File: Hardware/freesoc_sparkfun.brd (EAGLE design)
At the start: 116.8 x 55.9 mm, 92 parts, among them J1 5.5x2.1mm Barrel, U1 CY8C5888AXI-LP096, U2 AP2202-ADJ, U3 AP2202-ADJ, U4 AP2202-ADJ, U5 AP2202-ADJ, U6 AP2202-ADJ, U7 CY8C5868LTI-LP039

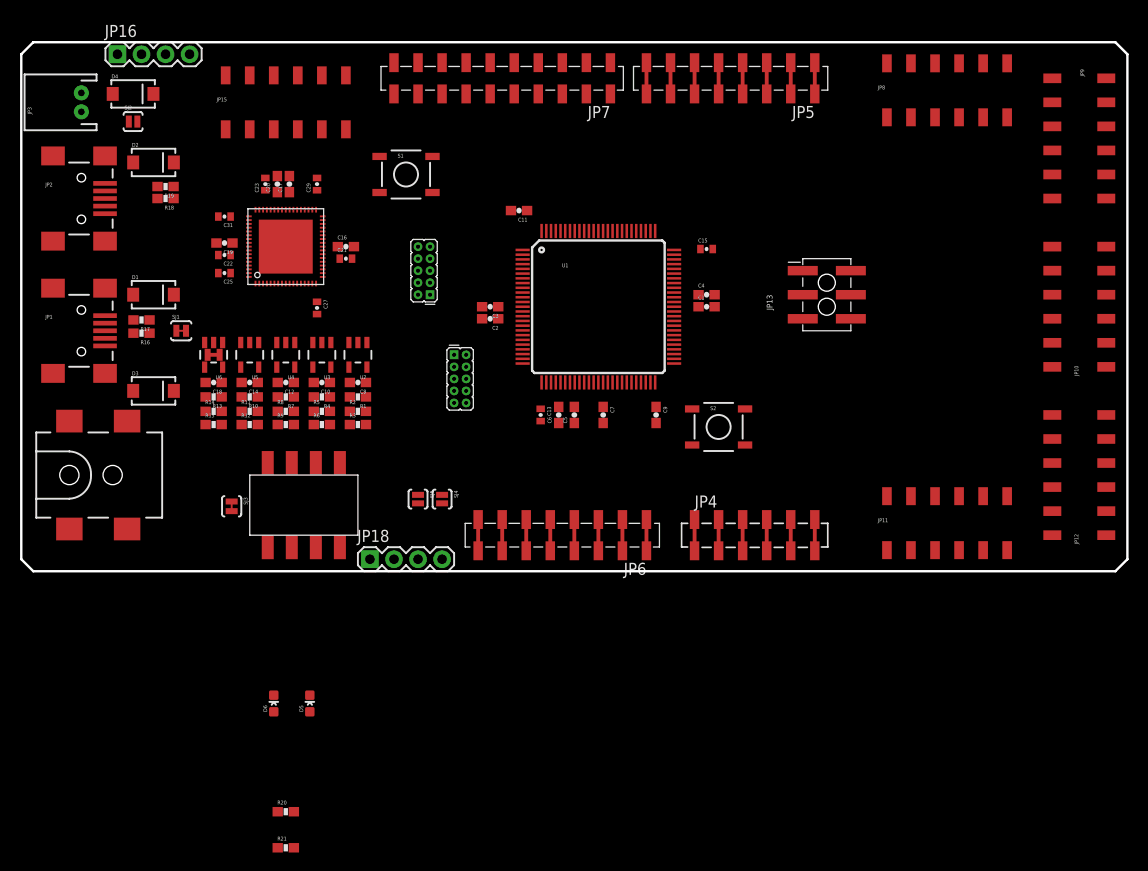
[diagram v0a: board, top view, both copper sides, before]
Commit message: Routed, ready for review.
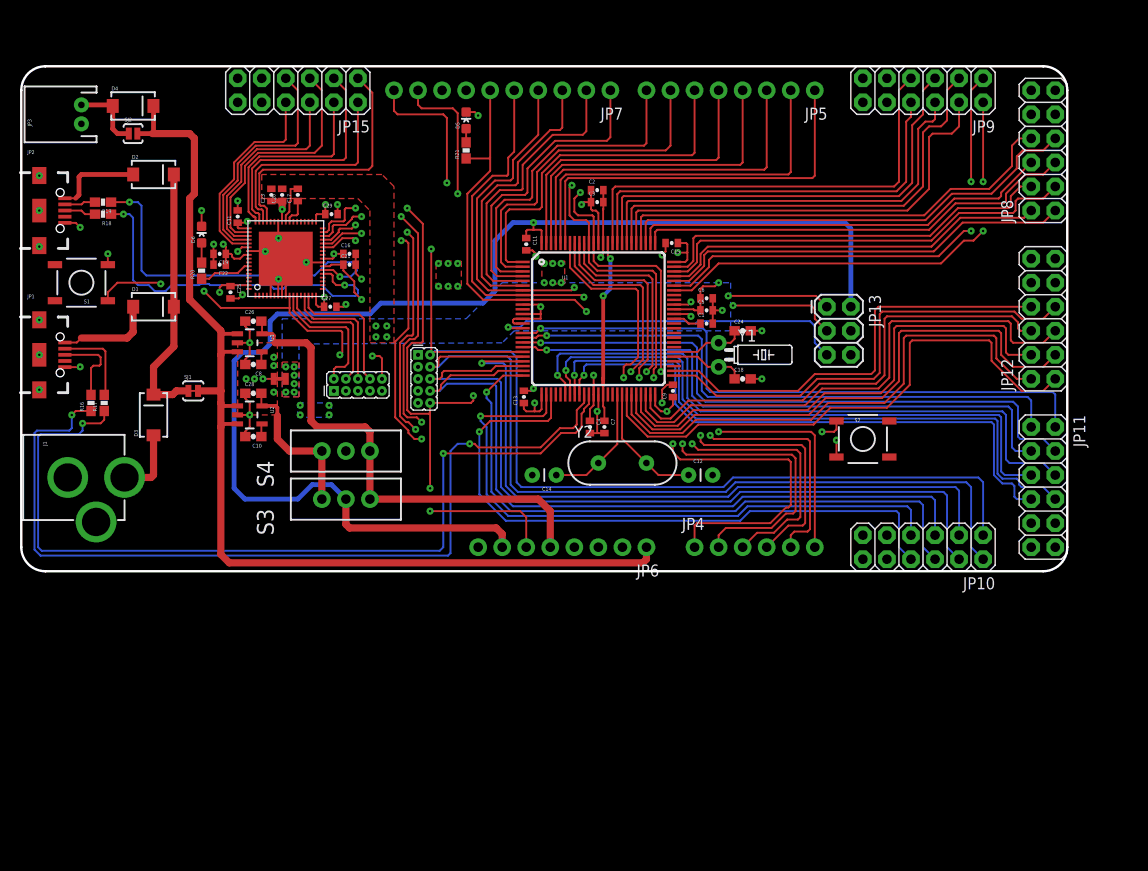
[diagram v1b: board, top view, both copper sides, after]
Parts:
- removed JP16, JP18: (no value), SparkFun-Connectors:1X04
- removed R1, R10, R13, R4, R7: 5.62k, SparkFun-Resistors:0603-RES
- removed R11, R14, R2, R5, R8: 3.40k, SparkFun-Resistors:0603-RES
- removed R12, R15, R3, R6, R9: 4.12k, SparkFun-Resistors:0603-RES
- removed SJ3: JUMPER-PAD-2-NC_BY_TRACE, SparkFun-Passives:PAD-JUMPER-2-NC_BY_TRACE_YES_SILK
- removed SJ4, SJ5: JUMPER-PAD-2-NOYES_SILK, SparkFun-Passives:PAD-JUMPER-2-NO_YES_SILK
- removed U$1: 4-POS-DIP, SparkFun-Electromechanical:4-POS-DIP-SMD
- removed U4, U5, U6: AP2202-ADJ, SparkFun-PowerIC:SOT23-5
- added C24: 22pF, SparkFun-Capacitors:0603-CAP
- added C26, C28: 2.2uF, SparkFun-Capacitors:0603-CAP
- added S3, S4: (no value), SparkFun-Electromechanical:SWITCH-SPDT
- added Y1: 32.768kHz, SparkFun-FreqCtrl:TC26H
- added Y2: (no value), SparkFun-FreqCtrl:HC49US
- C1, C11, C16, C17, C19, C2, C20, C3, C4, C5, C6, C7, C9: device SparkFun-Capacitors:0603-CAP -> SparkFun-Capacitors:0402-CAP
- C10, C8: value 2.2uF -> 470pF
- C12, C14: value 2.2uF -> (none); device SparkFun-Capacitors:0603-CAP -> SparkFun-Capacitors:CAP-PTH-SMALL
- C18: value 2.2uF -> 22pF
- J1: value 5.5x2.1mm Barrel -> POWER_JACKPTH; device SparkFun-Connectors:POWER_JACK_SMD -> SparkFun-Connectors:POWER_JACK_PTH
- JP1, JP2: value USBSMD -> MicroB; device SparkFun-Connectors:USB-MINIB -> SparkFun-Connectors:USB-B-MICRO-SMD_V03
- JP10, JP11, JP12, JP15, JP8, JP9: value M06X2FEMALE-SMT -> 2X6 FEMALE; device SparkFun-Connectors:2X6_SMD -> SparkFun-Connectors:2X6
- JP13: device SparkFun-Connectors:2X3_SMT_POSTS -> SparkFun-Connectors:2X3
- JP4: device SparkFun-Connectors:1X06_SMD_STRAIGHT_COMBO -> SparkFun-Connectors:1X06_NO_SILK
- JP5, JP6: device SparkFun-Connectors:1X08_SMD_COMBINED -> SparkFun-Connectors:1X08_NO_SILK
- JP7: value M10SMD_COMBO-FEMALE -> M10NO_SILK_PTH_FEMALE; device SparkFun-Connectors:1X10_SMD_COMBINED -> SparkFun-Connectors:1X10_NO_SILK
- U1: value CY8C5888AXI-LP096 -> CY8C5868AXI-LP035
- U2: value AP2202-ADJ -> MIC5219 5V
- U3: value AP2202-ADJ -> MIC5219 3.3V
- moved R21 76.1 mm to (47.0, 44.5), turned to 90 degrees
- moved D5 63.8 mm to (47.0, 47.6)
- moved R20 57.8 mm to (19.1, 31.8), turned to 90 degrees
- moved C18 55.9 mm to (76.2, 20.3), turned to 0 degrees
- moved D6 50.1 mm to (19.1, 35.6)
- moved C12 43.7 mm to (70.5, 10.2), turned to 0 degrees
- moved S1 36.1 mm to (6.35, 30.5), turned to 180 degrees
- moved C14 33.8 mm to (56.5, 10.2)
- moved JP10 25.0 mm to (101.6, 3.81), turned to 180 degrees
- moved C6 19.9 mm to (72.4, 28.8), turned to 0 degrees
- moved C4 18.6 mm to (60.1, 15.2), turned to 270 degrees
- moved JP8 18.0 mm to (109.2, 38.1), turned to 90 degrees
- moved C5 17.8 mm to (72.4, 27.6), turned to 0 degrees
- moved C2 17.7 mm to (60.8, 40.3), turned to 0 degrees
- moved JP14 16.9 mm to (39.4, 19.1), turned to 90 degrees
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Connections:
- net N$18 renamed PSOC_D+_PAD
- net N$19 renamed DEBUG_D-_PAD
- net N$22 renamed DEBUG_D+_PAD
- net N$3 renamed PSOC_D-_PAD
- removed net ADJ2: R1.2, R2.1, R3.1, U2.4
- removed net ADJ3: R4.2, R5.1, R6.1, U3.4
- removed net ADJ4: R7.2, R8.1, R9.1, U4.4
- removed net ADJ5: R10.2, R11.1, R12.1, U5.4
- removed net ADJ6: R13.2, R14.1, R15.1, U6.4
- removed net DEBUG_D+: JP2.D+, R18.2
- removed net DEBUG_D-: JP2.D-, R19.2
- removed net N$24: R20.1
- removed net N$31: SJ4.1, U7.38
- removed net N$32: SJ5.1, U7.39
- removed net PSOC_D+: JP1.D+, R16.2
- removed net PSOC_D-: JP1.D-, R17.2
- removed net SW2: R3.2, U$1.4
- removed net SW3: R6.2, U$1.3
- removed net SW4: R9.2, U$1.2
- removed net SW5: R12.2, U$1.1
- removed net SW6: R15.2, SJ3.1
- removed net VDDD/VDDA: C18.1, C19.1, C2.1, C20.1, C21.1, C22.1, C23.1, C25.1, C27.1, C3.1, C31.1, C4.1, C5.1, C6.1, JP14.1, JP15.10, JP15.9, JP16.2, JP6.4, JP6.5, R13.1, U1.37, U1.65, U1.88, U6.5, U7.17, U7.24, U7.44, U7.52, U7.59, U7.67
- removed net VDDIO_0: C14.1, C15.1, JP8.10, JP8.9, JP9.10, JP9.9, R10.1, U1.75, U5.5
- removed net VDDIO_1: C12.1, C13.1, C29.1, JP10.10, JP10.9, JP11.10, JP11.9, JP17.1, R7.1, U1.26, U4.5, U7.35
- removed net VDDIO_2: C10.1, C11.1, JP13.2, JP6.7, R4.1, U1.100, U3.5
- removed net VDDIO_3: C8.1, C9.1, JP12.10, JP12.9, JP18.2, R1.1, U1.50, U2.5
- new net 3.3V: C26.2, JP6.5, S3.3, S4.3, U3.5
- new net 5V: C20.1, C23.1, C28.2, C5.1, C6.1, JP6.4, S3.1, S4.1, U1.65, U2.5, U7.44
- new net DEBUG_D+_BUS: JP2.D+1, R18.2
- new net DEBUG_D-_BUS: JP2.D-1, R19.2
- new net DEBUG_LED: R20.1, U7.62
- new net N$1: C8.1, U3.4
- new net N$2: C10.1, U2.4
- new net PSOC_D+_BUS: JP1.D+1, R16.2
- new net PSOC_D-_BUS: JP1.D-1, R17.2
- new net VDDIO: C13.1, C15.1, C19.1, C2.1, C21.1, C22.1, C25.1, C27.1, C29.1, C3.1, C31.1, C4.1, C9.1, JP10.10, JP10.9, JP11.10, JP11.9, JP12.10, JP12.9, JP14.1, JP15.10, JP15.9, JP17.1, JP8.10, JP8.9, JP9.10, JP9.9, S4.2, U1.26, U1.37, U1.50, U1.75, U1.88, U7.17, U7.24, U7.35, U7.52, U7.59, U7.67
- new net VDDIO_ARDUINO: C11.1, JP13.2, JP6.7, S3.2, U1.100
- net A0: now also U1.94; no longer U1.89
- net A1: now also U1.93; no longer U1.90
- net A2: now also U1.92; no longer U1.91
- net A3: now also U1.91; no longer U1.92
- net A4: now also JP7.10, U1.90; no longer JP7.10A, JP7.10B, U1.93
- net A5: now also JP7.9, U1.89; no longer JP7.9A, JP7.9B, U1.94
- net AGND: now also C17.2, C20.2, C23.2, U7.43
- net D0: now also U1.95; no longer U1.99
- net D1: now also U1.96; no longer U1.1
- net D10: now also JP7.3, U1.6; no longer JP7.3A, JP7.3B, U1.2
- net D11: now also JP7.4, U1.7; no longer JP7.4A, JP7.4B, U1.8
- net D12: now also JP7.5, U1.8; no longer JP7.5A, JP7.5B, U1.7
- net D13: now also JP7.6; no longer JP7.6A, JP7.6B
- net D2: now also U1.97; no longer U1.98
- net D3: now also U1.98; no longer U1.5
- net D4: now also U1.99; no longer U1.95
- net D5: now also U1.1; no longer U1.6
- net D6: now also U1.2; no longer U1.3
- net D7: now also U1.3; no longer U1.97
- net D8: now also JP7.1, U1.4; no longer JP7.1A, JP7.1B, U1.96
- net D9: now also JP7.2, U1.5; no longer JP7.2A, JP7.2B, U1.4
- net DEBUG_I2C0_SCL: no longer JP16.4
- net DEBUG_I2C0_SDA: no longer JP16.3
- net GND: now also C24.2, C26.1, C28.1, J1.GNDBREAK, JP1.GND1, JP1.SHIELD1, JP1.SHIELD2, JP1.SHIELD3, JP2.GND1, JP2.SHIELD1, JP2.SHIELD2, JP2.SHIELD3, JP7.7; no longer C17.2, C20.2, C23.2, J1.P$4, JP1.GND, JP16.1, JP18.1, JP2.GND, JP7.7A, JP7.7B, R11.2, R14.2, R2.2, R5.2, R8.2, SJ3.2, U$1.5, U$1.6, U$1.7, U$1.8, U4.2, U5.2, U6.2, U7.43
- net N$13: now also J1.PWR; no longer J1.VIN0
- net N$15: now also JP1.VBUS1; no longer JP1.VBUS
- net P12.0: no longer JP18.4, SJ4.2
- net P12.1: no longer JP18.3, SJ5.2
- net P15.0: now also C14.1, Y2.1
- net P15.1: now also C12.1, Y2.2
- net P15.2: now also C18.1, Y1.2
- net P15.3: now also C24.1, Y1.1
- net P4.0: now also JP9.2; no longer JP9.1
- net P4.1: now also JP9.1; no longer JP9.2
- net P4.2: now also JP9.4; no longer JP9.3
- net P4.3: now also JP9.3; no longer JP9.4
- net P4.4: now also JP9.6; no longer JP9.5
- net P4.5: now also JP9.5; no longer JP9.6
- net P4.6: now also JP9.8; no longer JP9.7
- net P4.7: now also JP9.7; no longer JP9.8
- net P5.0: now also JP11.2; no longer JP11.1
- net P5.1: now also JP11.1; no longer JP11.2
- net P5.2: now also JP11.4; no longer JP11.3
- net P5.3: now also JP11.3; no longer JP11.4
- net P5.4: now also JP11.6; no longer JP11.5
- net P5.5: now also JP11.5; no longer JP11.6
- net P5.6: now also JP11.8; no longer JP11.7
- net P5.7: now also JP11.7; no longer JP11.8
- net V_DEBUG: now also JP2.VBUS1; no longer JP2.VBUS
- net V_IN: no longer U4.1, U4.3, U5.1, U5.3, U6.1, U6.3
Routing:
- net VDDIO_ARDUINO: track 0.00 -> 136.8 mm, vias 0 -> 1
- net P1.1: track 0.00 -> 134.1 mm, vias 0 -> 3
- net 5V: track 0.00 -> 131.4 mm, vias 0 -> 2
- net P1.3: track 0.00 -> 126.1 mm, vias 0 -> 3
- net !RESET: track 0.00 -> 125.0 mm, vias 0 -> 7
- net P1.4: track 0.00 -> 120.3 mm, vias 0 -> 3
- net P1.0: track 0.00 -> 112.0 mm, vias 0 -> 2
- net V_IN: track 0.00 -> 111.4 mm
- net GND: track 0.00 -> 97.7 mm, vias 0 -> 40
- net PSOC_D+_PAD: track 0.00 -> 93.5 mm, vias 0 -> 2
- net PSOC_D-_PAD: track 0.00 -> 93.3 mm, vias 0 -> 2
- net A4: track 0.00 -> 92.4 mm, vias 0 -> 4
- net A5: track 0.00 -> 88.8 mm, vias 0 -> 4
- net P1.2: track 0.00 -> 73.4 mm, vias 0 -> 1
- net P1.7: track 0.00 -> 68.6 mm, vias 0 -> 1
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- added copper zone on layer 1, net AGND
- added copper zone on layer 16, net AGND
- added copper zone on layer 1, net GND
- added copper zone on layer 15, net GND
- added copper zone on layer 1, net VDDIO
- added copper zone on layer 16, net VDDIO
- added copper zone on layer 2, net VDDIO
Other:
- board size 116.8 x 55.9 mm -> 110.5 x 53.3 mm
